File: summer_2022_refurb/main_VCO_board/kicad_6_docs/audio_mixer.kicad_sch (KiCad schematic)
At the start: 14 parts

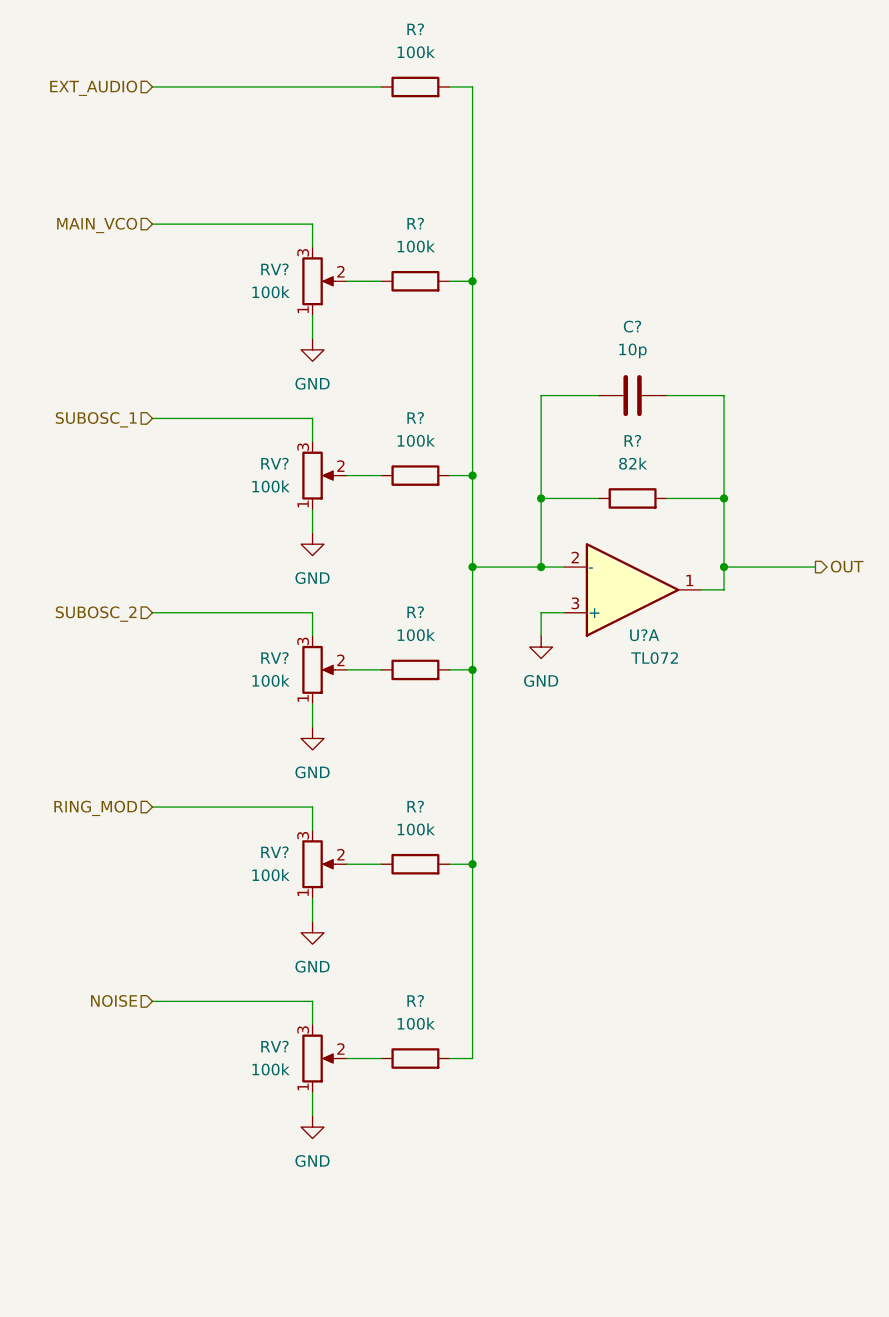
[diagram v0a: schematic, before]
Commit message: Main VCO progress
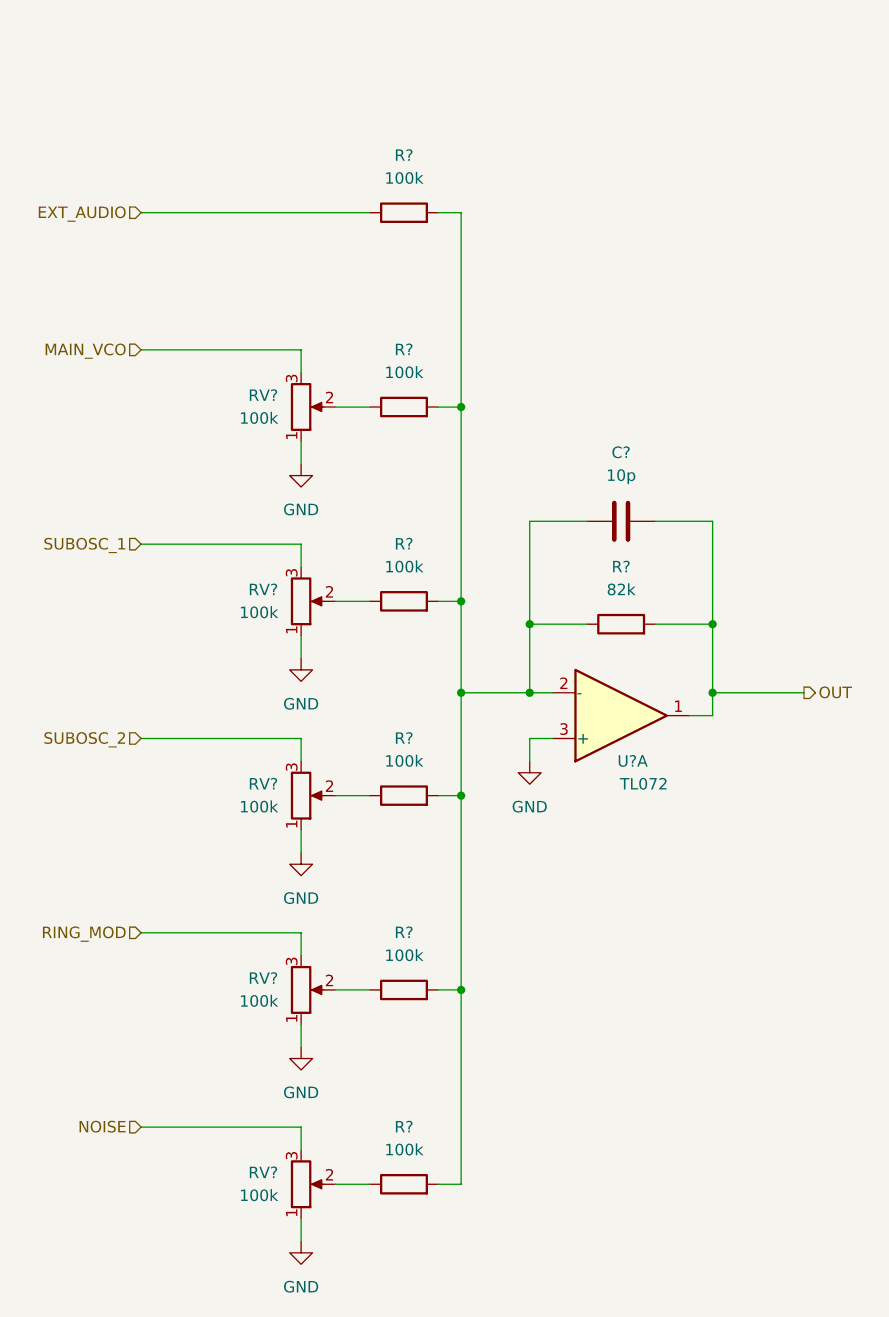
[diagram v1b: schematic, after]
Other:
- title: (none) -> Josh Ox Ribon Synth Main VCO board
- moved on the sheet: C?, R?, RV?, U?A
